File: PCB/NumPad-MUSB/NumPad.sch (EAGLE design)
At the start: 125 parts, among them J1 J, J10 J, J11 J, J12 J, J13 J, J14 J, J15 J, J16 J, J17 J, J2 J, J3 J, J4 J, J5 J, J6 J, J7 J, J8 J, J9 J

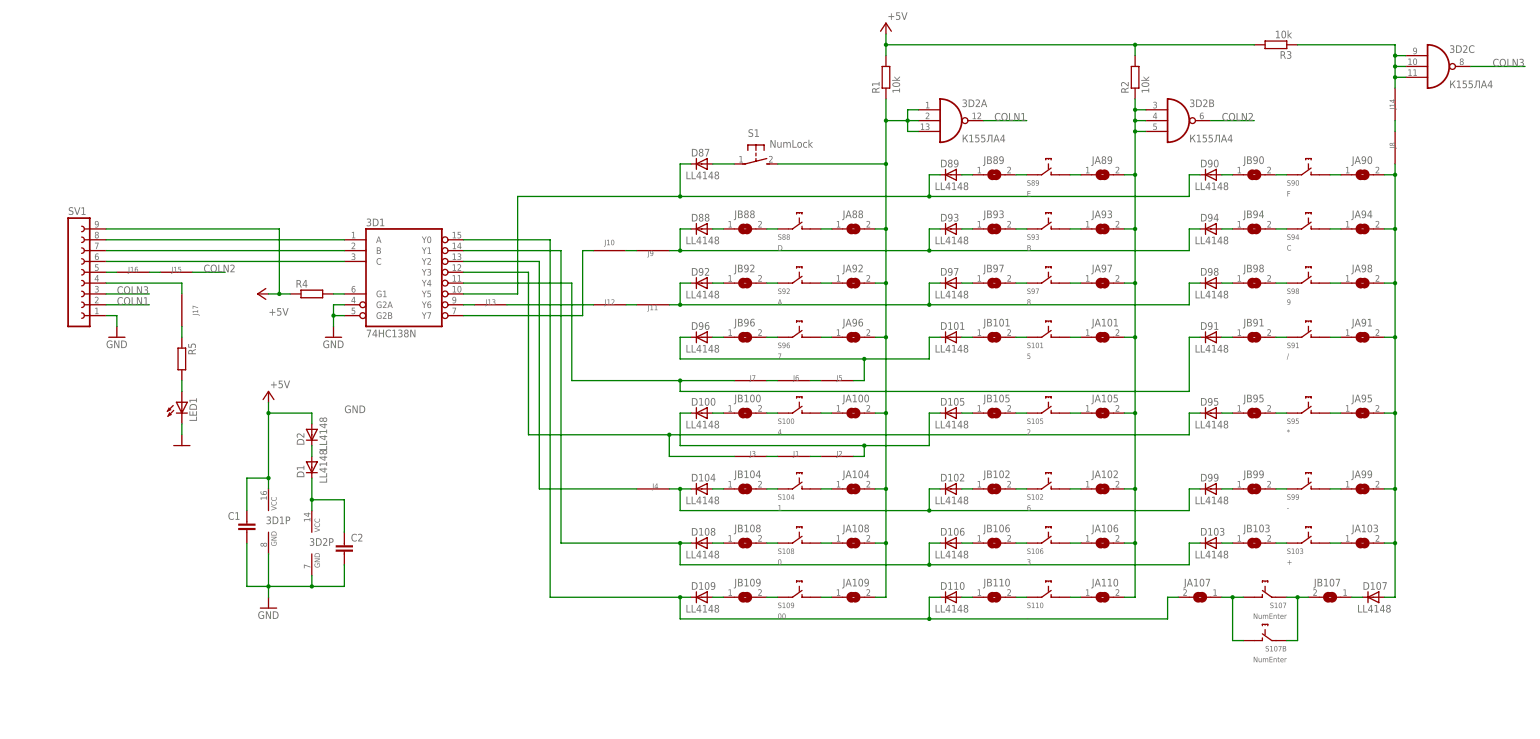
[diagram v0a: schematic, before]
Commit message: get all vil
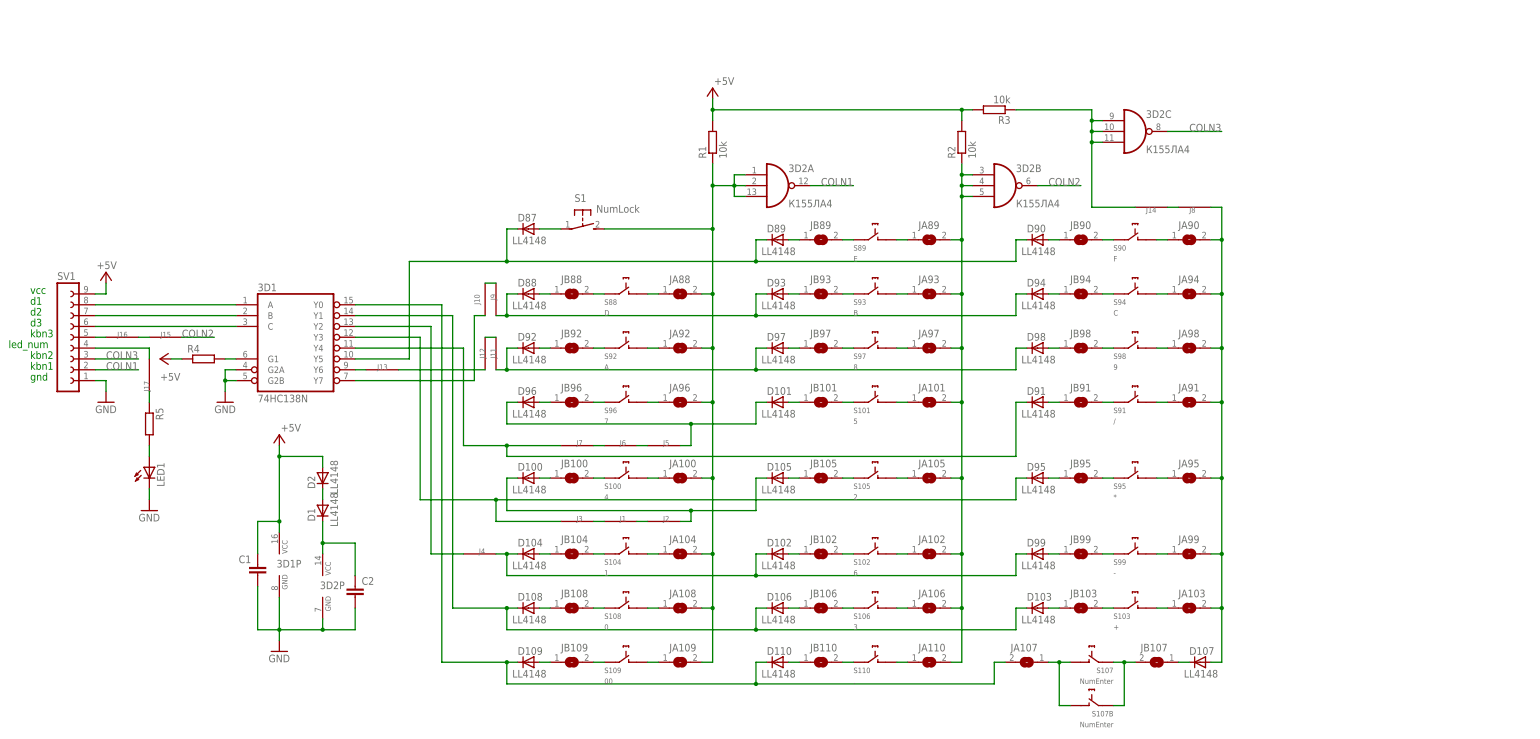
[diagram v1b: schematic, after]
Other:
- note added: "d1"
- note added: "d2"
- note added: "d3"
- note added: "gnd"
- note added: "kbn1"
- note added: "kbn2"
- note added: "kbn3"
- note added: "led_num"
- note added: "vcc"
- moved on the sheet: 3D1, 3D1P, 3D2A, 3D2B, 3D2C, 3D2P, C1, C2, D1, D100, D101, D102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
